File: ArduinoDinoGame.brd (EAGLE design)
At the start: 120.8 x 86 mm, 15 parts, among them U1 ARDUINO-UNO-R3-SHIELD

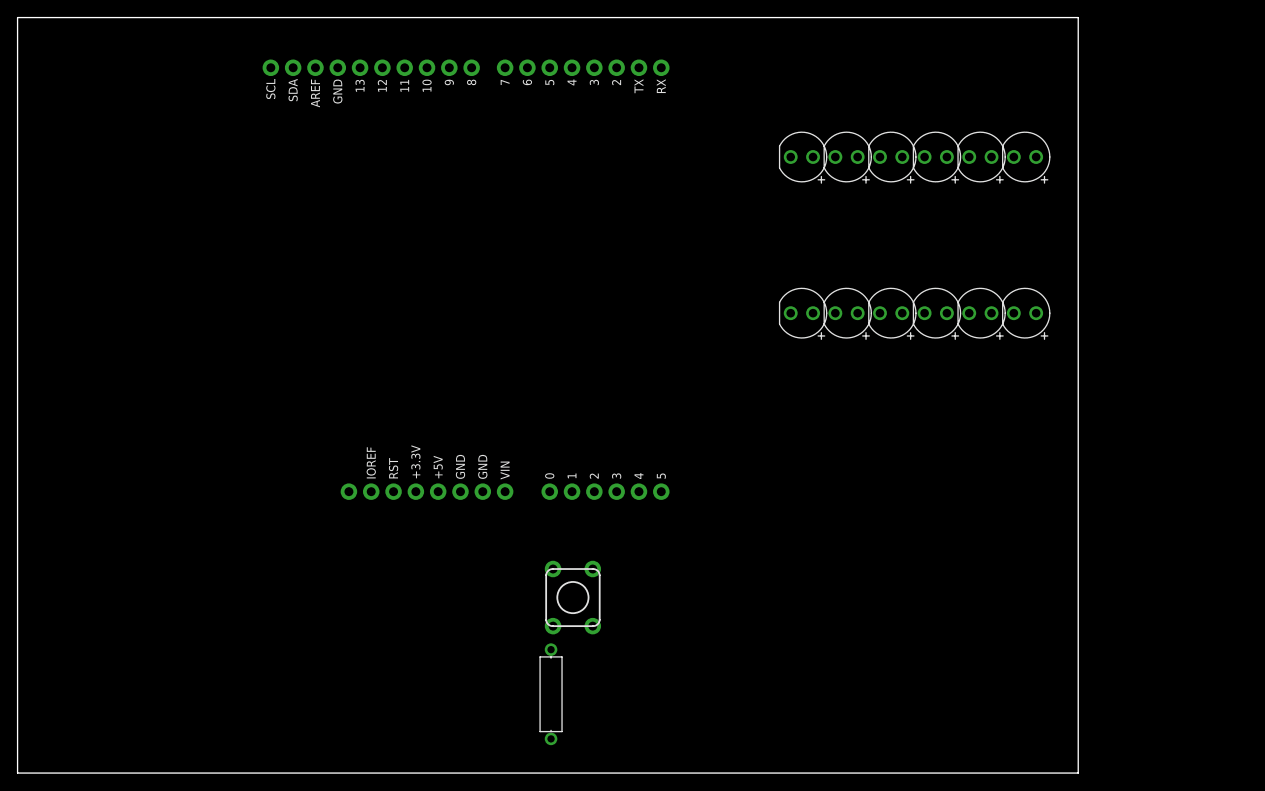
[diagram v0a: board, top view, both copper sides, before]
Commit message: Update ArduinoDinoGame.brd
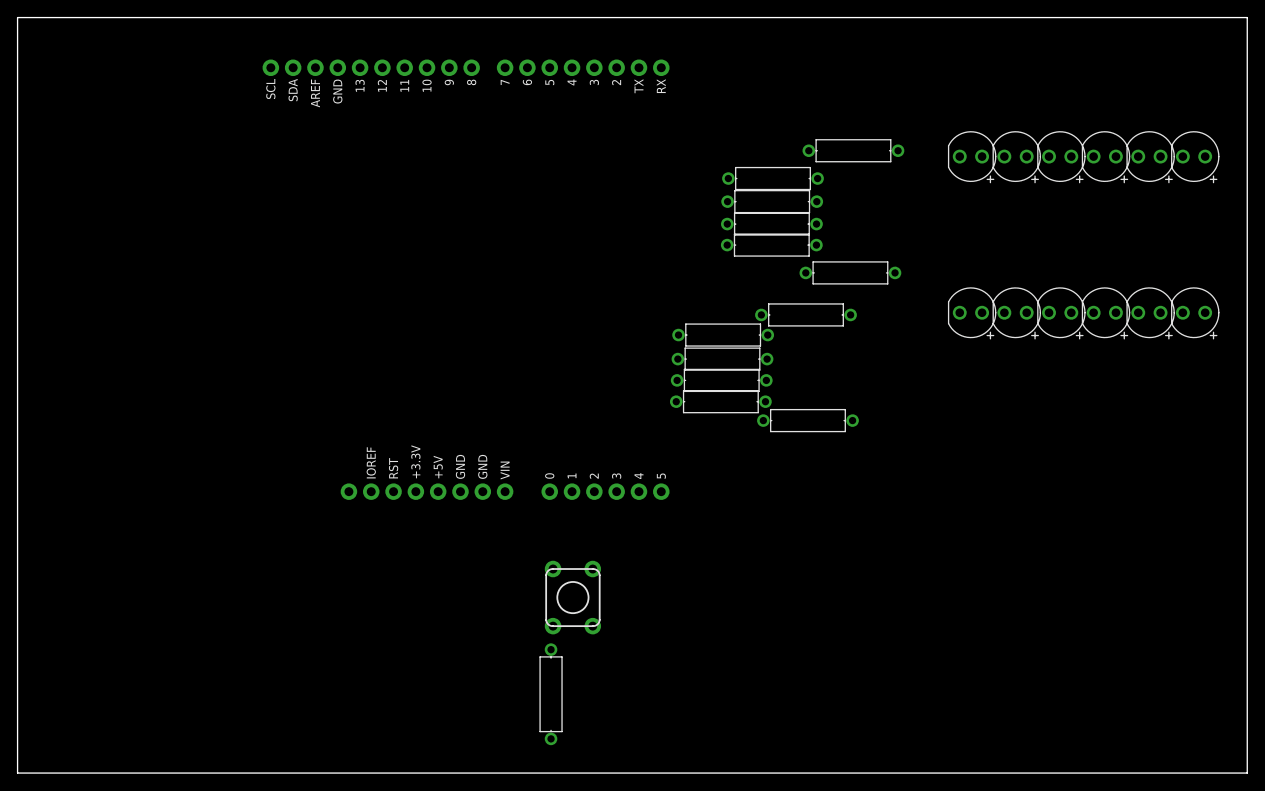
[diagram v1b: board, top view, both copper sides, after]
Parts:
- added R10, R11, R12, R13, R14, R3, R4, R5, R6, R7, R8, R9: 150, Tinkercad:RESAD1016W63L850D250B
- moved D1 19.2 mm to (108.5, 70.2)
- moved D10 19.2 mm to (123.8, 70.2)
- moved D11 19.2 mm to (113.6, 52.4)
- moved D12 19.2 mm to (118.7, 52.4)
- moved D14 19.2 mm to (123.8, 52.4)
- moved D2 19.2 mm to (108.5, 52.4)
- moved D4 19.2 mm to (113.6, 70.2)
- moved D6 19.2 mm to (133.9, 52.4)
- moved D7 19.2 mm to (118.7, 70.2)
- moved D8 19.2 mm to (133.9, 70.2)
- moved D3 19.2 mm to (128.9, 52.4)
- moved D5 19.2 mm to (128.9, 70.2)
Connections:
- new net D10_A: D10.1, R10.2
- new net D11_A: D11.1, R4.2
- new net D12_A: D12.1, R5.2
- new net D14_A: D14.1, R6.2
- new net D1_A: D1.1, R9.2
- new net D2_A: D2.1, R3.2
- new net D3_A: D3.1, R7.2
- new net D4_A: D4.1, R14.2
- new net D5_A: D5.1, R11.2
- new net D6_A: D6.1, R8.2
- new net D7_A: D7.1, R13.2
- new net D8_A: D8.1, R12.2
- net U1_D10: now also R13.1; no longer D7.1
- net U1_D11: now also R10.1; no longer D10.1
- net U1_D12: now also R11.1; no longer D5.1
- net U1_D13: now also R12.1; no longer D8.1
- net U1_D2: now also R3.1; no longer D2.1
- net U1_D3: now also R4.1; no longer D11.1
- net U1_D4: now also R5.1; no longer D12.1
- net U1_D5: now also R6.1; no longer D14.1
- net U1_D6: now also R7.1; no longer D3.1
- net U1_D7: now also R8.1; no longer D6.1
- net U1_D8: now also R9.1; no longer D1.1
- net U1_D9: now also R14.1; no longer D4.1
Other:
- board size 120.8 x 86 mm -> 140 x 86 mm
